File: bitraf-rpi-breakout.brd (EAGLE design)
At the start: 65.7 x 57.1 mm, 20 parts, among them IC1 74HC595N, K1 JS-M1-9V-4, T1 BC547

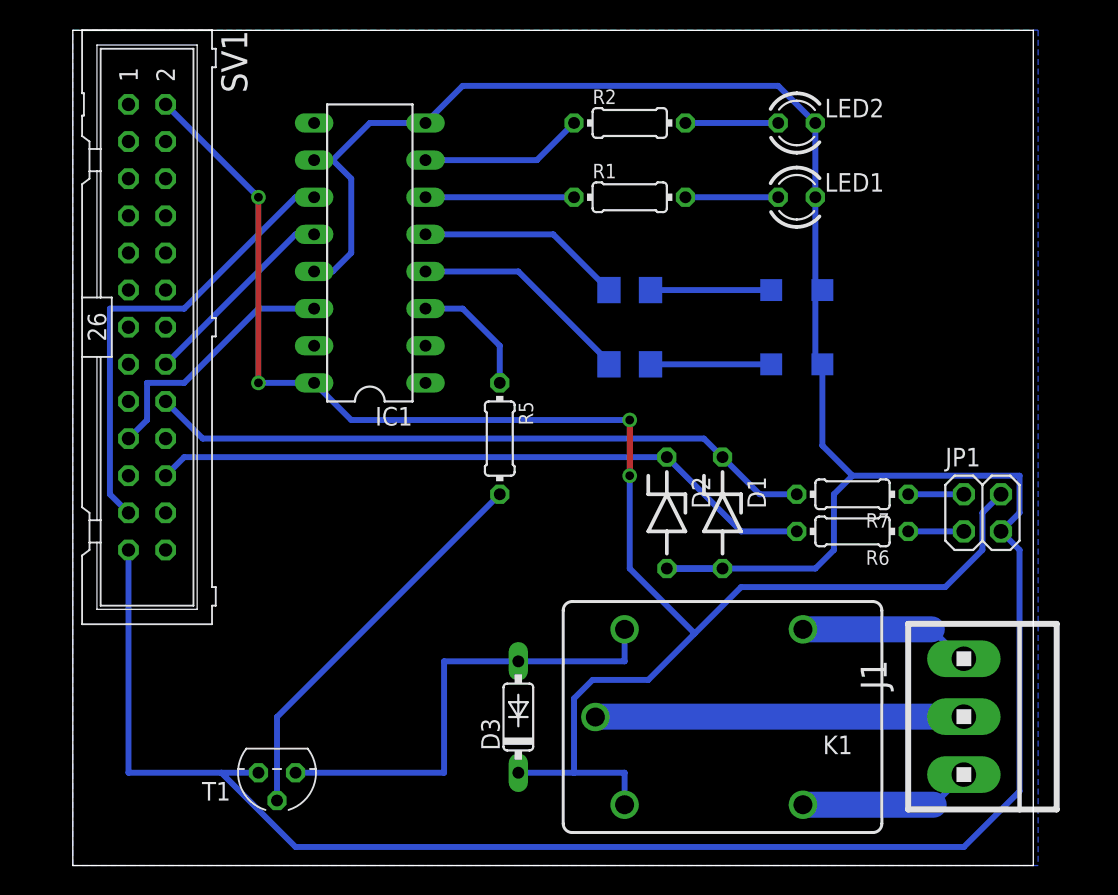
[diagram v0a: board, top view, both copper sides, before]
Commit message: Rev b.
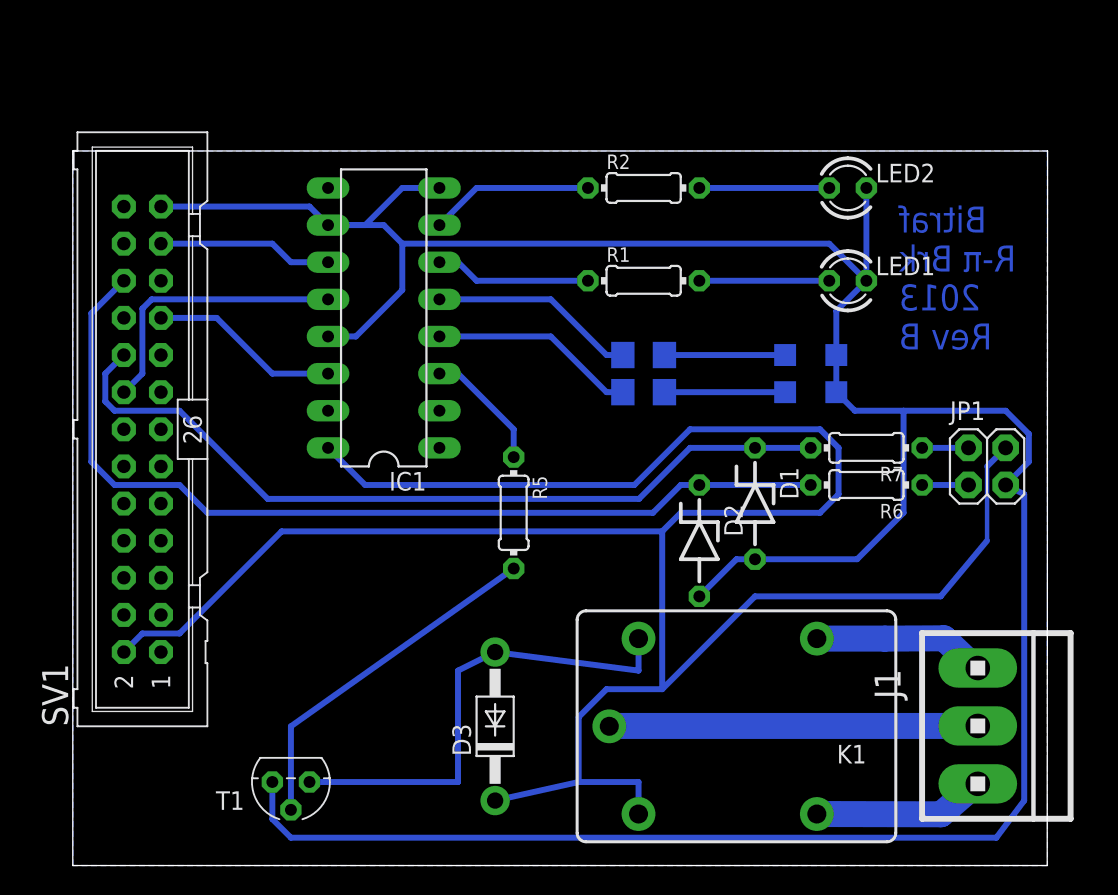
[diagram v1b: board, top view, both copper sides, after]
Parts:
- D1, D2: value (none) -> 3.3V
- D3: value 1N4148DO35-7 -> 1N4004; device diode:DO35-7 -> diode:DO41-10
- R1, R2, R3, R4: value (none) -> 330
- R6, R7: value (none) -> 4.7k
- moved SV1 6.99 mm to (4.76, 29.8), turned to 90 degrees
- moved LED1 6.70 mm to (53.0, 40.0)
- moved R1 5.79 mm to (39.1, 40.0)
- moved LED2 5.65 mm to (53.0, 46.4)
- moved R5 5.17 mm to (30.2, 24.1)
- moved LED3 4.55 mm to (50.5, 34.9)
- moved R2 4.55 mm to (39.1, 46.4)
- moved R4 4.55 mm to (39.1, 34.9)
- moved IC1 4.55 mm to (21.3, 37.5)
- moved R6 3.31 mm to (54.3, 26.0)
- moved R7 3.31 mm to (54.3, 28.6)
- moved JP1 3.19 mm to (62.5, 27.3)
- moved D2 2.93 mm to (42.9, 22.2)
- moved D1 2.31 mm to (46.7, 24.8)
- moved LED4 2.13 mm to (50.5, 32.4)
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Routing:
- net VCC: track 115.6 -> 162.0 mm, vias 4 -> 0
- net N$20: track 31.6 -> 12.0 mm
- net N$8: track 45.8 -> 64.8 mm
- net N$9: track 45.8 -> 56.2 mm
- net GND: track 211.2 -> 203.4 mm
- net N$19: track 13.8 -> 19.2 mm
- net N$21: track 17.9 -> 13.0 mm
- net N$6: track 27.3 -> 24.4 mm
- net N$2: track 6.35 -> 8.89 mm
- net N$1: track 6.35 -> 8.89 mm
- net N$12: track 15.3 -> 14.1 mm
- net TTL_IN_2: track 3.81 -> 3.18 mm
- net TTL_IN_1: track 3.81 -> 3.18 mm
- net N$5: track 10.2 -> 10.7 mm
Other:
- board size 65.7 x 57.1 mm -> 66.7 x 48.9 mm
- board text added: "Bitraf R-π Brk 2013 Rev B"
